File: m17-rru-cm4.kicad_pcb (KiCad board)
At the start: 2 copper layers, 1 part, among them U1 Compute_Module_4_Connectors

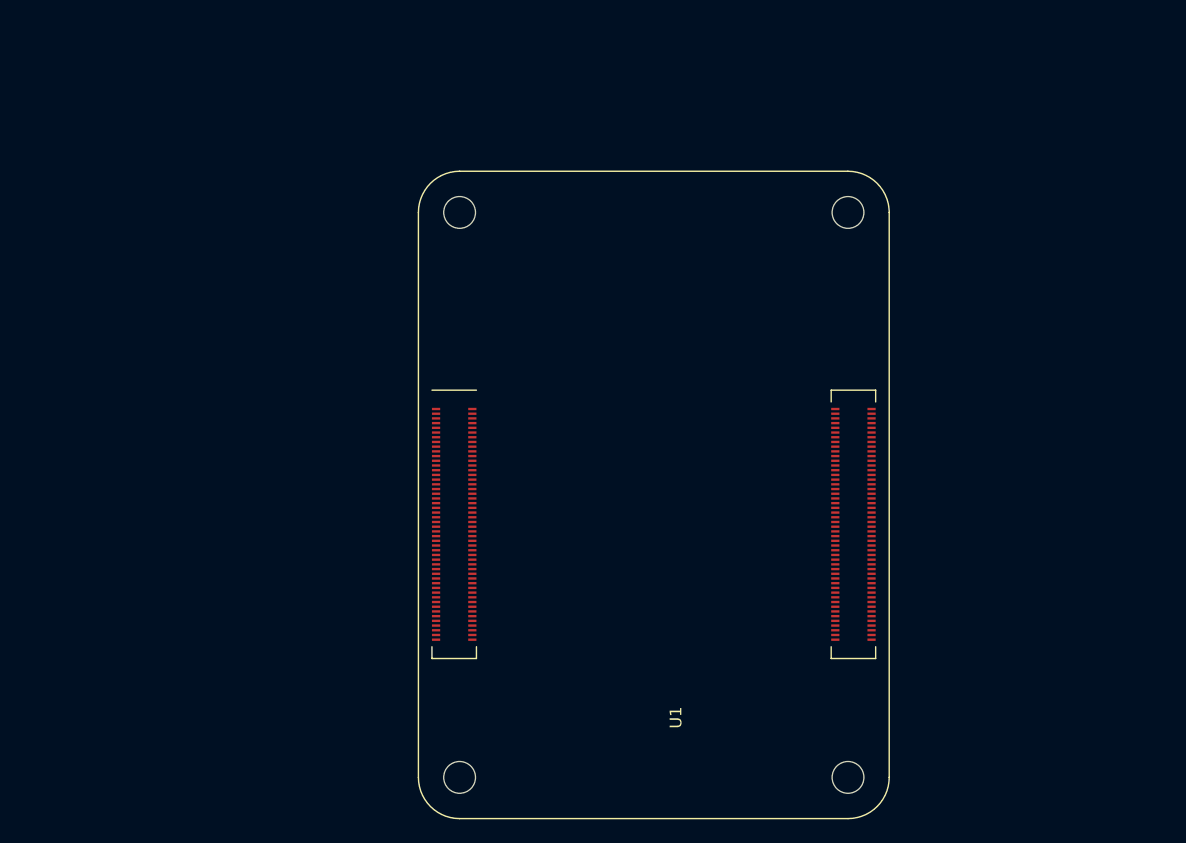
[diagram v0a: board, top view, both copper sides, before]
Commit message: WIP PCB
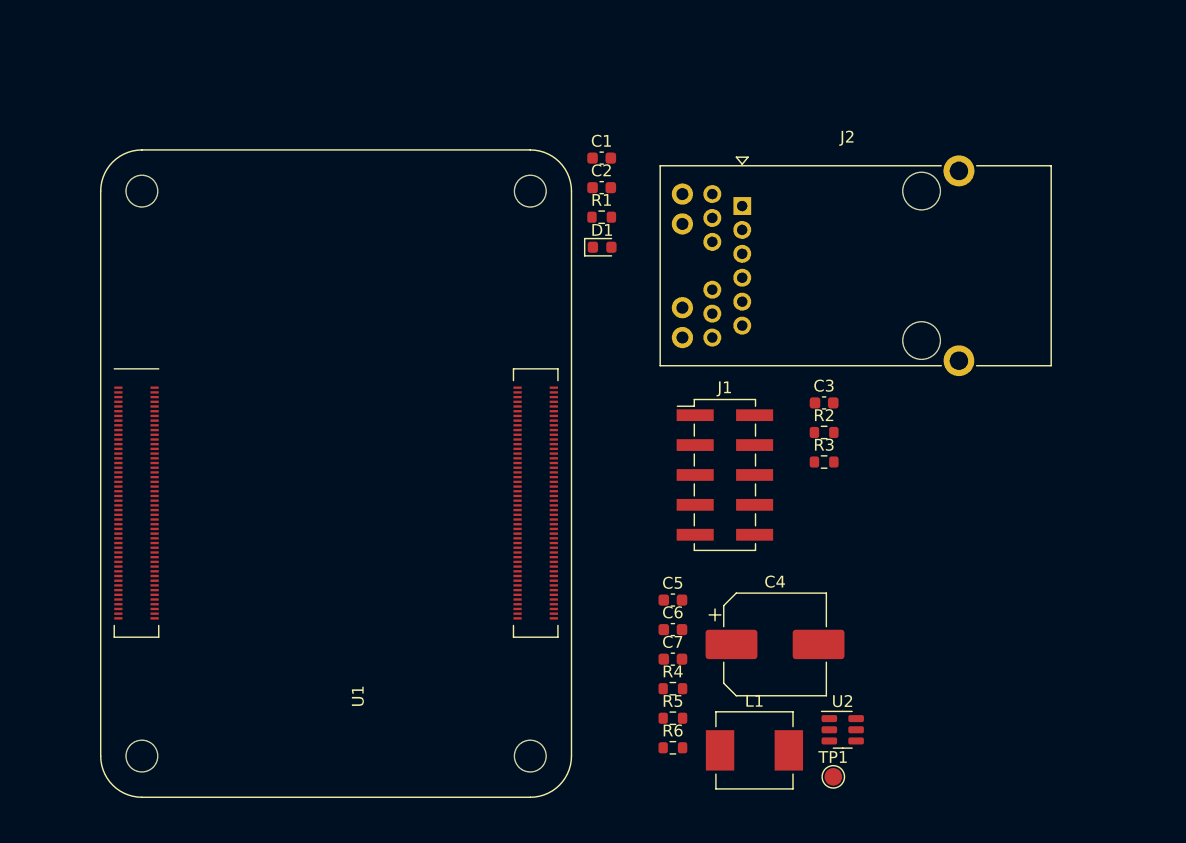
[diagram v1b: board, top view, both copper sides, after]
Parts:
- added C1: 100n, Capacitor_SMD:C_0603_1608Metric, F.Cu at (149.1, 71.4)
- added C2: 100n, Capacitor_SMD:C_0603_1608Metric, F.Cu at (149.1, 73.9)
- added C3: 100n, Capacitor_SMD:C_0603_1608Metric, F.Cu at (168.0, 92.2)
- added C4: 100u/50V, Capacitor_SMD:CP_Elec_8x10.5, F.Cu at (163.8, 112.7)
- added C5: 100n, Capacitor_SMD:C_0603_1608Metric, F.Cu at (155.1, 108.9)
- added C6: 100n, Capacitor_SMD:C_0603_1608Metric, F.Cu at (155.1, 111.4)
- added C7: 22u/6.3V, Capacitor_SMD:C_0603_1608Metric, F.Cu at (155.1, 114.0)
- added D1: LED GRN, LED_SMD:LED_0603_1608Metric, F.Cu at (149.1, 79.0)
- added J1: Conn_02x05_Odd_Even, Connector_PinHeader_2.54mm:PinHeader_2x05_P2.54mm_Vertical_SMD, F.Cu at (159.5, 98.3)
- added J2: RJ45_JK0654219, Connector_RJ:RJ45_Pulse_JK0654219NL_Horizontal, F.Cu at (161.0, 75.5)
- added L1: 10u, Inductor_SMD:L_Vishay_IHLP-2525, F.Cu at (162.1, 121.7)
- added R1: 470R, Resistor_SMD:R_0603_1608Metric, F.Cu at (149.1, 76.4)
- added R2: 470R, Resistor_SMD:R_0603_1608Metric, F.Cu at (168.0, 94.7)
- added R3: 470R, Resistor_SMD:R_0603_1608Metric, F.Cu at (168.0, 97.2)
- added R4: 100k, Resistor_SMD:R_0603_1608Metric, F.Cu at (155.1, 116.5)
- added R5: 24k, Resistor_SMD:R_0603_1608Metric, F.Cu at (155.1, 119.0)
- added R6: 126k, Resistor_SMD:R_0603_1608Metric, F.Cu at (155.1, 121.5)
- added TP1: TP, TestPoint:TestPoint_Pad_D1.5mm, F.Cu at (168.8, 124.0)
- added U2: TP6841, Package_TO_SOT_SMD:SOT-23-6, F.Cu at (169.6, 120.0)
- U1: value Compute_Module_4_Connectors -> Compute Module 4
- moved U1 27.1 mm to (126.5, 100.7)
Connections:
- U1 pad 1: unconnected-(U1A-GND-Pad1) -> GND
- U1 pad 10: unconnected-(U1A-Ethernet_Pair0_N-Pad10) -> /CM4 module/ETH_0N
- U1 pad 107: unconnected-(U1B-GND-Pad107) -> GND
- U1 pad 108: unconnected-(U1B-GND-Pad108) -> GND
- U1 pad 11: unconnected-(U1A-Ethernet_Pair2_P-Pad11) -> /CM4 module/ETH_2P
- U1 pad 113: unconnected-(U1B-GND-Pad113) -> GND
- U1 pad 114: unconnected-(U1B-GND-Pad114) -> GND
- U1 pad 119: unconnected-(U1B-GND-Pad119) -> GND
- U1 pad 12: unconnected-(U1A-Ethernet_Pair0_P-Pad12) -> /CM4 module/ETH_0P
- U1 pad 120: unconnected-(U1B-GND-Pad120) -> GND
- U1 pad 125: unconnected-(U1B-GND-Pad125) -> GND
- U1 pad 126: unconnected-(U1B-GND-Pad126) -> GND
- U1 pad 13: unconnected-(U1A-GND-Pad13) -> GND
- U1 pad 131: unconnected-(U1B-GND-Pad131) -> GND
- U1 pad 132: unconnected-(U1B-GND-Pad132) -> GND
- U1 pad 137: unconnected-(U1B-GND-Pad137) -> GND
- U1 pad 138: unconnected-(U1B-GND-Pad138) -> GND
- U1 pad 14: unconnected-(U1A-GND-Pad14) -> GND
- U1 pad 144: unconnected-(U1B-GND-Pad144) -> GND
- U1 pad 15: unconnected-(U1A-~{Ethernet_nLED3}-Pad15) -> /CM4 module/ETH_LEDY
- U1 pad 150: unconnected-(U1B-GND-Pad150) -> GND
- U1 pad 155: unconnected-(U1B-GND-Pad155) -> GND
- U1 pad 156: unconnected-(U1B-GND-Pad156) -> GND
- U1 pad 161: unconnected-(U1B-GND-Pad161) -> GND
- U1 pad 162: unconnected-(U1B-GND-Pad162) -> GND
- U1 pad 167: unconnected-(U1B-GND-Pad167) -> GND
- U1 pad 168: unconnected-(U1B-GND-Pad168) -> GND
- U1 pad 17: unconnected-(U1A-~{Ethernet_nLED2}-Pad17) -> /CM4 module/ETH_LEDG
- U1 pad 173: unconnected-(U1B-GND-Pad173) -> GND
- U1 pad 174: unconnected-(U1B-GND-Pad174) -> GND
- U1 pad 179: unconnected-(U1B-GND-Pad179) -> GND
- U1 pad 180: unconnected-(U1B-GND-Pad180) -> GND
- U1 pad 185: unconnected-(U1B-GND-Pad185) -> GND
- U1 pad 186: unconnected-(U1B-GND-Pad186) -> GND
- U1 pad 191: unconnected-(U1B-GND-Pad191) -> GND
- U1 pad 192: unconnected-(U1B-GND-Pad192) -> GND
- U1 pad 197: unconnected-(U1B-GND-Pad197) -> GND
- U1 pad 198: unconnected-(U1B-GND-Pad198) -> GND
- U1 pad 2: unconnected-(U1A-GND-Pad2) -> GND
- U1 pad 21: unconnected-(U1A-~{Pi_nLED_Activity}-Pad21) -> Net-(D1-K)
- U1 pad 22: unconnected-(U1A-GND-Pad22) -> GND
- U1 pad 23: unconnected-(U1A-GND-Pad23) -> GND
- U1 pad 3: unconnected-(U1A-Ethernet_Pair3_P-Pad3) -> /CM4 module/ETH_3P
- U1 pad 32: unconnected-(U1A-GND-Pad32) -> GND
- U1 pad 33: unconnected-(U1A-GND-Pad33) -> GND
- U1 pad 4: unconnected-(U1A-Ethernet_Pair1_P-Pad4) -> /CM4 module/ETH_1P
- U1 pad 42: unconnected-(U1A-GND-Pad42) -> GND
- U1 pad 43: unconnected-(U1A-GND-Pad43) -> GND
- U1 pad 48: unconnected-(U1A-GPIO27-Pad48) -> /CM4 module/BOOT0
- U1 pad 49: unconnected-(U1A-GPIO18-Pad49) -> /CM4 module/PA_EN
- U1 pad 5: unconnected-(U1A-Ethernet_Pair3_N-Pad5) -> /CM4 module/ETH_3N
- U1 pad 50: unconnected-(U1A-GPIO17-Pad50) -> /CM4 module/~{RST}
- U1 pad 51: unconnected-(U1A-GPIO15-Pad51) -> /CM4 module/UART_RX
- U1 pad 52: unconnected-(U1A-GND-Pad52) -> GND
- U1 pad 53: unconnected-(U1A-GND-Pad53) -> GND
- U1 pad 55: unconnected-(U1A-GPIO14-Pad55) -> /CM4 module/UART_TX
- U1 pad 59: unconnected-(U1A-GND-Pad59) -> GND
- U1 pad 6: unconnected-(U1A-Ethernet_Pair1_N-Pad6) -> /CM4 module/ETH_1N
- U1 pad 60: unconnected-(U1A-GND-Pad60) -> GND
- U1 pad 65: unconnected-(U1A-GND-Pad65) -> GND
- U1 pad 66: unconnected-(U1A-GND-Pad66) -> GND
- U1 pad 7: unconnected-(U1A-GND-Pad7) -> GND
- U1 pad 71: unconnected-(U1A-GND-Pad71) -> GND
- U1 pad 74: unconnected-(U1A-GND-Pad74) -> GND
- U1 pad 77: unconnected-(U1A-+5V-Pad77) -> /CM4 module/5V
- U1 pad 78: unconnected-(U1A-GPIO_VREF-Pad78) -> +3.3V
- U1 pad 79: unconnected-(U1A-+5V-Pad79) -> /CM4 module/5V
- U1 pad 8: unconnected-(U1A-GND-Pad8) -> GND
- U1 pad 81: unconnected-(U1A-+5V-Pad81) -> /CM4 module/5V
- U1 pad 83: unconnected-(U1A-+5V-Pad83) -> /CM4 module/5V
- U1 pad 84: unconnected-(U1A-CM4_3.3V_Out-Pad84) -> +3.3V
- U1 pad 85: unconnected-(U1A-+5V-Pad85) -> /CM4 module/5V
- U1 pad 86: unconnected-(U1A-CM4_3.3V_Out-Pad86) -> +3.3V
- U1 pad 87: unconnected-(U1A-+5V-Pad87) -> /CM4 module/5V
- U1 pad 9: unconnected-(U1A-Ethernet_Pair2_N-Pad9) -> /CM4 module/ETH_2N
- U1 pad 98: unconnected-(U1A-GND-Pad98) -> GND

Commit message: WIP PCB layout
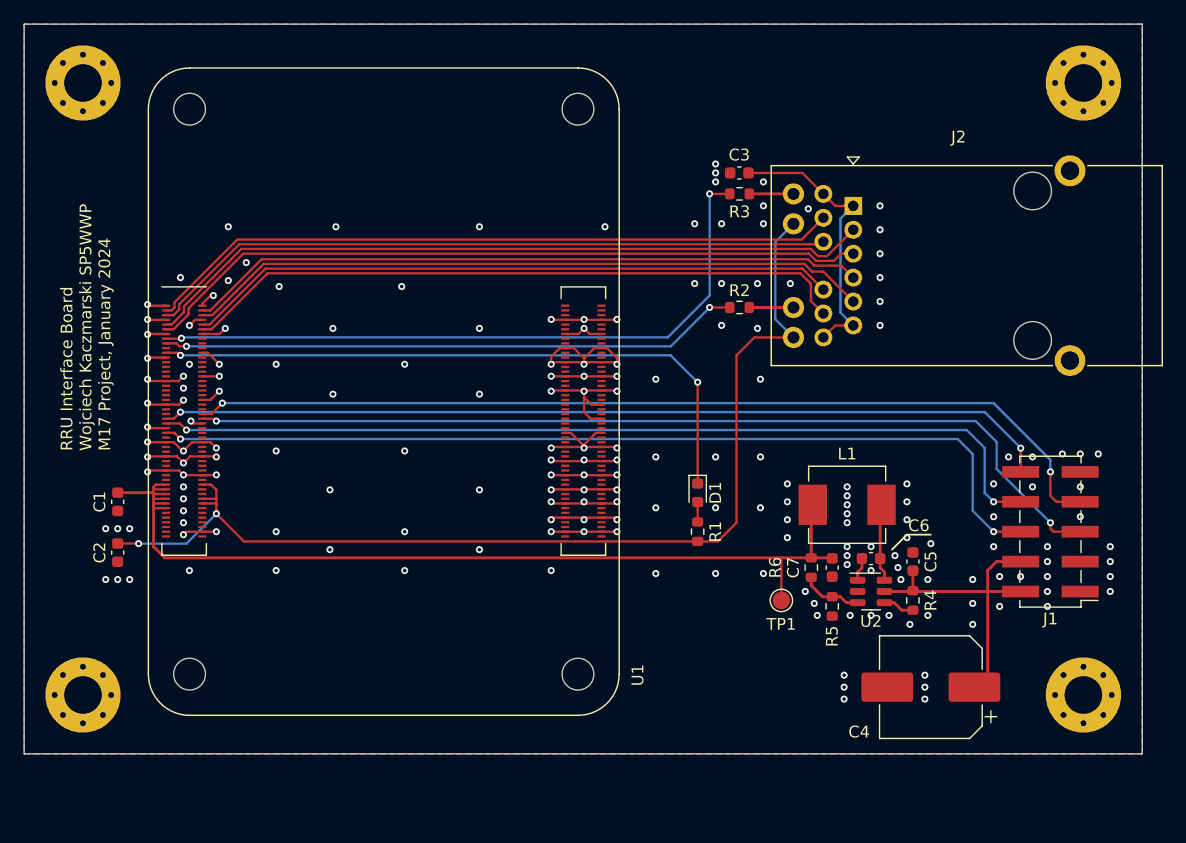
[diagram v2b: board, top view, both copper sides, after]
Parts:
- added H1: MountingHole_Pad, MountingHole:MountingHole_3.2mm_M3_Pad_Via, F.Cu at (105.0, 117.0)
- added H2: MountingHole_Pad, MountingHole:MountingHole_3.2mm_M3_Pad_Via, F.Cu at (190.0, 117.0)
- added H3: MountingHole_Pad, MountingHole:MountingHole_3.2mm_M3_Pad_Via, F.Cu at (190.0, 65.0)
- added H4: MountingHole_Pad, MountingHole:MountingHole_3.2mm_M3_Pad_Via, F.Cu at (105.0, 65.0)
- moved C2 51.5 mm to (108.0, 104.9), turned to -90 degrees
- moved C1 50.4 mm to (108.0, 100.6), turned to -90 degrees
- moved J1 28.1 mm to (187.2, 103.1), turned to 180 degrees
- moved R1 27.9 mm to (157.2, 103.1), turned to 90 degrees
- moved R3 23.9 mm to (160.8, 74.4)
- moved D1 22.4 mm to (157.2, 99.8), turned to -90 degrees
- moved L1 22.3 mm to (169.9, 100.8), turned to 180 degrees
- moved R4 21.7 mm to (175.5, 109.0), turned to -90 degrees
- moved C3 20.8 mm to (160.8, 72.6), turned to 180 degrees
- moved C5 20.7 mm to (175.5, 105.7), turned to 90 degrees
- moved R6 19.3 mm to (166.9, 106.2), turned to 90 degrees
- moved C6 17.9 mm to (172.0, 105.4)
- moved R5 16.5 mm to (168.7, 109.5), turned to -90 degrees
- moved TP1 15.6 mm to (164.3, 109.0)
- moved C7 15.6 mm to (168.7, 106.2), turned to 90 degrees
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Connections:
- R2 pad 1: /CM4 module/ETH_LEDY -> /CM4 module/ETH_LEDG
- R3 pad 1: /CM4 module/ETH_LEDG -> /CM4 module/ETH_LEDY
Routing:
- net GND: track 0.00 -> 132.1 mm, vias 0 -> 195
- net +3.3V: track 0.00 -> 91.8 mm, vias 0 -> 2
- net /CM4 module/5V: track 0.00 -> 81.0 mm
- net /CM4 module/BOOT0: track 0.00 -> 80.2 mm, vias 0 -> 2
- net /CM4 module/~{RST}: track 0.00 -> 80.2 mm, vias 0 -> 2
- net /CM4 module/UART_TX: track 0.00 -> 78.9 mm, vias 0 -> 2
- net /CM4 module/UART_RX: track 0.00 -> 77.6 mm, vias 0 -> 2
- net /CM4 module/PA_EN: track 0.00 -> 76.1 mm, vias 0 -> 2
- net /CM4 module/ETH_2N: track 0.00 -> 62.5 mm
- net /CM4 module/ETH_2P: track 0.00 -> 61.9 mm
- net /CM4 module/ETH_3P: track 0.00 -> 59.4 mm
- net /CM4 module/ETH_3N: track 0.00 -> 58.7 mm
- net /CM4 module/ETH_1N: track 0.00 -> 58.4 mm
- net /CM4 module/ETH_LEDY: track 0.00 -> 58.1 mm, vias 0 -> 2
- net /CM4 module/ETH_1P: track 0.00 -> 57.8 mm
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- added copper zone on B.Cu, net GND
- added copper zone on F.Cu, net GND
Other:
- board outline added: 95 x 62 mm
- board text added: "RRU Interface Board Wojciech Kaczmarski SP5WWP M17 Project, January 2024"
